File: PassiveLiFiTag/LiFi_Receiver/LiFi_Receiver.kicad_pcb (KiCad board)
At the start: 2 copper layers, 180.6 x 107.8 mm, 58 parts, among them J1 Conn_01x07, J2 Conn_01x02, J3 Conn_01x02, J4 Conn_01x02, J5 Conn_01x02, SW1 SW_Push, U1 MSP430FR5994IPNR, U10 ADG721BRMZ-REEL, U11 S-1313B24-M5T1U3, U2 TS881ILT, U3 BQ25570RGRR, U4 HDC2080DMBR, U5 HDC2080DMBR, U6 ADG722BRMZ-REEL7, U7 ADG722BRMZ-REEL7, U8 ADG721BRMZ-REEL, U9 ADG721BRMZ-REEL, Y1 Crystal_Small

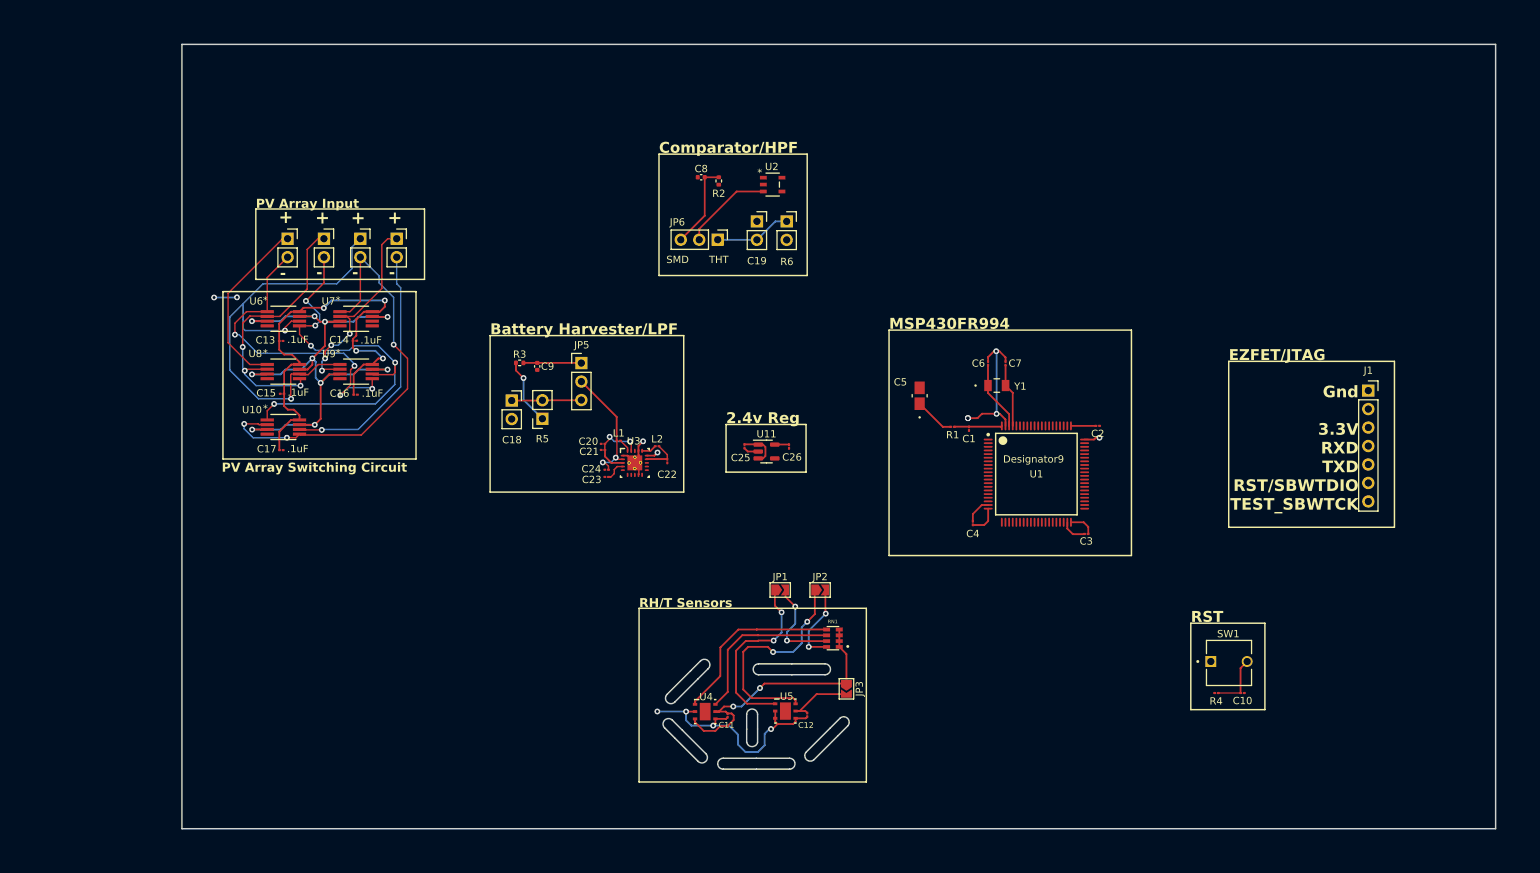
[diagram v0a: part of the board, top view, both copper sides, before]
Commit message: Design almost completed
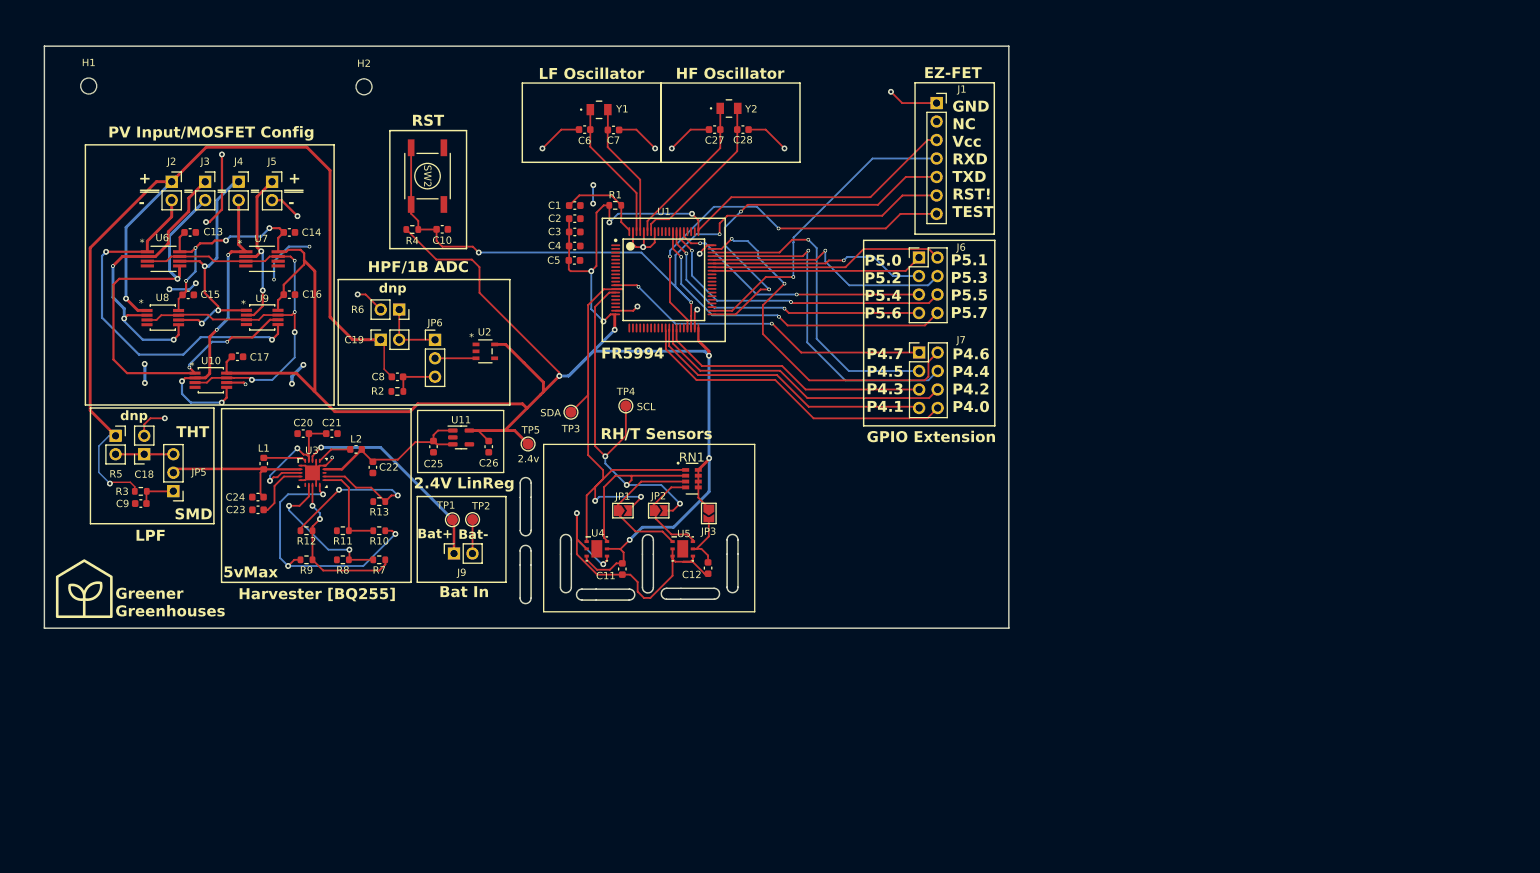
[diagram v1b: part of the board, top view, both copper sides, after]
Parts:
- removed SW1: SW_Push, LIFI-FOOTPRINTS:SW_TL59NF160Q
- added C27: DNP, Capacitor_SMD:C_0603_1608Metric, F.Cu at (138.4, 45.5)
- added C28: DNP, Capacitor_SMD:C_0603_1608Metric, F.Cu at (142.3, 45.5)
- added H1: MountingHole, MountingHole:MountingHole_2.2mm_M2, F.Cu at (52.3, 39.5)
- added H2: MountingHole, MountingHole:MountingHole_2.2mm_M2, F.Cu at (90.2, 39.6)
- added J6: Conn_01x08, Connector_PinHeader_2.54mm:PinHeader_2x04_P2.54mm_Vertical, F.Cu at (166.5, 63.1)
- added J7: Conn_01x08, Connector_PinHeader_2.54mm:PinHeader_2x04_P2.54mm_Vertical, F.Cu at (166.5, 76.2)
- added J9: Conn_01x02, Connector_PinSocket_2.54mm:PinSocket_1x02_P2.54mm_Vertical, F.Cu at (102.5, 103.8)
- added R10: R_Small_US, Resistor_SMD:R_0603_1608Metric, F.Cu at (92.3, 100.6)
- added R11: R_Small_US, Resistor_SMD:R_0603_1608Metric, F.Cu at (87.3, 100.6)
- added R12: R_Small_US, Resistor_SMD:R_0603_1608Metric, F.Cu at (82.3, 100.6)
- added R13: R_Small_US, Resistor_SMD:R_0603_1608Metric, F.Cu at (92.3, 96.6)
- added R7: R_Small_US, Resistor_SMD:R_0603_1608Metric, F.Cu at (92.3, 104.6)
- added R8: R_Small_US, Resistor_SMD:R_0603_1608Metric, F.Cu at (87.3, 104.6)
- added R9: R_Small_US, Resistor_SMD:R_0603_1608Metric, F.Cu at (82.3, 104.6)
- added SW2: PTS645SL43SMTR92LFS, Library:PTS645SL43SMTR92LFS_CNK-M, F.Cu at (98.9, 51.9)
- added TP1: TestPoint, TestPoint:TestPoint_Pad_D1.5mm, F.Cu at (102.3, 99.1)
- added TP2: TestPoint, TestPoint:TestPoint_Pad_D1.5mm, F.Cu at (105.1, 99.1)
- added TP3: SDA, TestPoint:TestPoint_Pad_D1.5mm, F.Cu at (118.6, 84.4)
- added TP4: SCL, TestPoint:TestPoint_Pad_D1.5mm, F.Cu at (126.2, 83.5)
- added TP5: 2.4v, TestPoint:TestPoint_Pad_D1.5mm, F.Cu at (112.7, 88.7)
- added Y2: Crystal_Small, Library:xtal-2, F.Cu at (140.3, 42.6)
- C1, C10, C11, C12, C13, C14, C15, C16, C17, C2, C20, C21, C22, C23, C24, C25, C26, C3, C4, C6, C7: footprint Capacitor_SMD:C_01005_0402Metric -> Capacitor_SMD:C_0603_1608Metric
- C5: footprint LIFI-FOOTPRINTS:TAJA_AVX-M -> Capacitor_SMD:C_0603_1608Metric
- C8, C9: footprint Capacitor_SMD:C_0402_1005Metric -> Capacitor_SMD:C_0603_1608Metric
- L1, L2: footprint Inductor_SMD:L_01005_0402Metric -> Inductor_SMD:L_0603_1608Metric
- R1, R4: footprint Resistor_SMD:R_01005_0402Metric -> Resistor_SMD:R_0603_1608Metric
- R2, R3: footprint Resistor_SMD:R_0402_1005Metric -> Resistor_SMD:R_0603_1608Metric
- RN1: footprint LIFI-FOOTPRINTS:Res_network -> Library:RESCAV80P320X160X70-8N
- U10, U8, U9: footprint LIFI-FOOTPRINTS:RM_8_ADI-M -> Library:RM_8_ADI
- U2: footprint LIFI-FOOTPRINTS:TS88_3 -> Library:SOT23-5_TS881_TEX
- U3: footprint Library:Bat_Harv2 -> Library:Bat_Harv1
- U4, U5: footprint LIFI-FOOTPRINTS:HDC2080_1 -> Library:DMB0006A_NV
- U6, U7: footprint LIFI-FOOTPRINTS:RM_8_ADI-M -> Library:RM_8_ADI-M
- moved R4 127.6 mm to (96.8, 59.2)
- moved C10 127.2 mm to (100.9, 59.2)
- moved C3 81.7 mm to (119.1, 59.6), turned to 0 degrees
- moved C2 77.3 mm to (119.1, 57.7)
- moved J1 71.3 mm to (168.9, 41.9)
- moved C4 66.7 mm to (119.1, 61.5), turned to 0 degrees
- moved Y1 66.5 mm to (122.5, 42.8)
- moved C6 64.1 mm to (120.5, 45.5), turned to 0 degrees
- moved C7 62.7 mm to (124.5, 45.6), turned to 180 degrees
- moved C1 62.3 mm to (119.1, 55.9), turned to 0 degrees
- moved JP5 58.8 mm to (64.0, 95.2), turned to 180 degrees
- moved R5 58.7 mm to (56.0, 87.6), turned to 0 degrees
- moved U1 57.8 mm to (131.4, 66.2)
- moved C9 57.7 mm to (59.5, 96.9), turned to 180 degrees
- moved R1 55.5 mm to (124.7, 55.9)
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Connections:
- J1 pad 3: +3.3V -> VCC
- JP1 pad 1: sda2 -> UCB2SDA_BYP
- JP1 pad 2: Net-(JP1-B) -> UCB2SDA
- JP2 pad 1: Net-(JP2-A) -> UCB2SCL_BYP
- JP2 pad 2: scl2 -> UCB2SCL
- RN1 pad 1: (no net) -> UCB2SDA
- RN1 pad 2: (no net) -> UCB2SCL
- RN1 pad 3: (no net) -> UCB2SDA_BYP
- RN1 pad 4: VCC -> UCB2SCL_BYP
- RN1 pad 5: Net-(JP1-B) -> VCC
- RN1 pad 6: (no net) -> VCC
- RN1 pad 7: (no net) -> VCC
- RN1 pad 8: (no net) -> VCC
- U1 pad 12: unconnected-(U1-P4.7-Pad12) -> Net-(J7-Pin_1)
- U1 pad 31: unconnected-(U1-P4.0_A8-Pad31) -> Net-(J7-Pin_8)
- U1 pad 32: unconnected-(U1-P4.1_A9-Pad32) -> Net-(J7-Pin_7)
- U1 pad 33: unconnected-(U1-P4.2_A10-Pad33) -> Net-(J7-Pin_6)
- U1 pad 34: unconnected-(U1-P4.3_A11-Pad34) -> Net-(J7-Pin_5)
- U1 pad 53: unconnected-(U1-P5.0_UCB1SIMO_UCB1SDA-Pad53) -> Net-(J6-Pin_1)
- U1 pad 54: unconnected-(U1-P5.1_UCB1SOMI_UCB1SCL-Pad54) -> Net-(J6-Pin_2)
- U1 pad 55: unconnected-(U1-P5.2_UCB1CLK_TA4CLK-Pad55) -> Net-(J6-Pin_3)
- U1 pad 56: unconnected-(U1-P5.3_UCB1STE-Pad56) -> Net-(J6-Pin_4)
- U1 pad 57: unconnected-(U1-P4.4_TB0.5-Pad57) -> Net-(J7-Pin_4)
- U1 pad 58: unconnected-(U1-P4.5-Pad58) -> Net-(J7-Pin_3)
- U1 pad 59: unconnected-(U1-P4.6-Pad59) -> Net-(J7-Pin_2)
- U1 pad 65: unconnected-(U1-P5.4_UCA2TXD_UCA2SIMO_TB0OUTH-Pad65) -> Net-(J6-Pin_5)
- U1 pad 66: unconnected-(U1-P5.5_UCA2RXD_UCA2SOMI_ACLK-Pad66) -> Net-(J6-Pin_6)
- U1 pad 67: unconnected-(U1-P5.6_UCA2CLK_TA4.0_SMCLK-Pad67) -> Net-(J6-Pin_7)
- U1 pad 68: unconnected-(U1-P5.7_UCA2STE_TA4.1_MCLK-Pad68) -> Net-(J6-Pin_8)
- U1 pad 74: unconnected-(U1-PJ.6_HFXIN-Pad74) -> Net-(U1-PJ.6_HFXIN)
- U1 pad 75: unconnected-(U1-PJ.7_HFXOUT-Pad75) -> Net-(U1-PJ.7_HFXOUT)
- U11 pad 4: (no net) -> unconnected-(U11-NC-Pad4)
- U3 pad 5: unconnected-(U3-EN_N-Pad5) -> GND
- U4 pad 1: Net-(U4-SDA) -> UCB2SDA
- U4 pad 6: Net-(U4-SCL) -> UCB2SCL
- U5 pad 1: Net-(U5-SDA) -> UCB2SDA_BYP
- U5 pad 6: Net-(U5-SCL) -> UCB2SCL_BYP
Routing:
- net VCC: track 118.1 -> 354.3 mm, vias 6 -> 13
- net P1+: track 33.9 -> 136.7 mm, vias 1 -> 2
- net ~{RST}/SBWTDIO_N: track 7.79 -> 105.5 mm, vias 0 -> 3
- net UCB2SCL: track 0.00 -> 70.1 mm, vias 0 -> 3
- net UCB2SDA: track 0.00 -> 69.5 mm, vias 0 -> 2
- net GND: track 108.7 -> 162.8 mm, vias 14 -> 28
- net TEST_SBWTCK: track 0.00 -> 53.0 mm, vias 0 -> 2
- net P2.0_UART_TXD: track 0.00 -> 52.1 mm, vias 0 -> 2
- net Net-(J7-Pin_2): track 0.00 -> 51.0 mm, vias 0 -> 2
- net Net-(J7-Pin_4): track 0.00 -> 46.7 mm, vias 0 -> 1
- net Net-(J6-Pin_8): track 0.00 -> 46.2 mm, vias 0 -> 2
- net Net-(J7-Pin_1): track 0.00 -> 45.8 mm, vias 0 -> 2
- net Net-(J7-Pin_8): track 0.00 -> 44.5 mm
- net Net-(J7-Pin_3): track 0.00 -> 43.8 mm, vias 0 -> 1
- net Net-(J6-Pin_6): track 0.00 -> 42.7 mm, vias 0 -> 2
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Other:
- board size 180.6 x 107.8 mm -> 132.6 x 80 mm
- board text added: "2.4V LinReg"
- board text added: "2.4v"
- board text added: "5vMax"
- board text added: "Bat In"
- board text added: "Bat+"
- board text added: "Bat-"
- board text added: "EZ-FET"
- board text added: "FR5994"
- board text added: "GND NC Vcc RXD TXD RST! TEST"
- board text added: "GPIO Extension"
- board text added: "Greener Greenhouses"
- board text added: "HF Oscillator"
- board text added: "HPF/1B ADC"
- board text added: "Harvester [BQ255]"
- board text added: "LF Oscillator"
- board text added: "LPF"
- board text added: "P4.6 P4.4 P4.2 P4.0"
- board text added: "P4.7 P4.5 P4.3 P4.1"
- board text added: "P5.0 P5.2 P5.4 P5.6"
- board text added: "P5.1 P5.3 P5.5 P5.7"
- board text added: "PV Input/MOSFET Config"
- board text added: "SCL"
- board text added: "SDA"
- board text added: "U3"
- board text added: "Y1"
- board text added: "Y2"
- board text added: "dnp"
- board text removed: "2.4v Reg"
- board text removed: "Battery Harvester/LPF"
- board text removed: "Comparator/HPF"
- board text removed: "EZFET/JTAG"
- board text removed: "Gnd 3.3V RXD TXD RST/SBWTDIO TEST_SBWTCK"
- board text removed: "MSP430FR994"
- board text removed: "PV Array Input"
- board text removed: "PV Array Switching Circuit"
